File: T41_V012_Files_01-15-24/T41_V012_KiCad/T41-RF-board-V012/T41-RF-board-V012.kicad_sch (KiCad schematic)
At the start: 224 parts, among them J1 IQ_Out, J2 RF_IN, J3 RFControl, J4 12-13.8V, J5 IQ_In, J6 RF_OUT, Q1 BS170, U1 74CBTLV3253DR, U10 SN74LVC1G04DCK, U106 MC33078, U107 MC33078, U11 Si5351A-B-GT, U12 PE4312, U13 MAR-3SM+, U14 LM7805CT, U15 LM1117T-3.3, U16 MC33078, U17 LM317L, U18 SN74LVC1G04DCK, U19 MASWSS0179, U2 PSA-8A+, U20 MASWSS0179, U21 MCP23017_SO, U22 HMC434E, U23 HMC434E, U3 PE4312, U4 74CBTLV3253DR, U5 SN74LVC1G04DCK, U6 MC33078, U7 MASWSS0179, U8 MC33078, U9 MASWSS0179, Y1 ECS-TX053-S3, Y2 25MHz

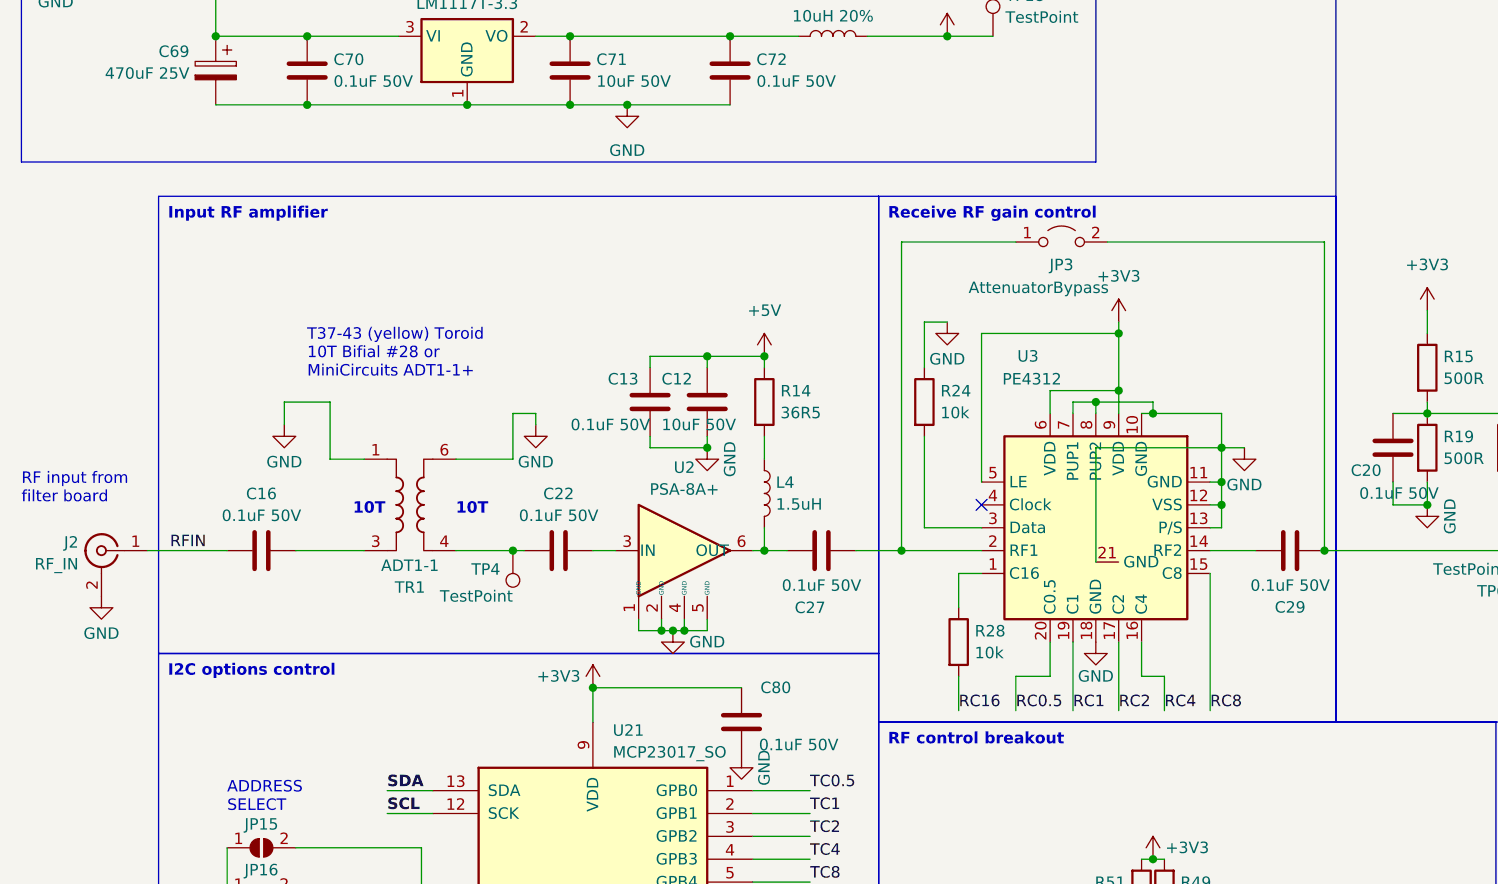
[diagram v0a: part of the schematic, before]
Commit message: Switched order of attenuator and amplifier in receive chain. Now attenuator is before amplifier
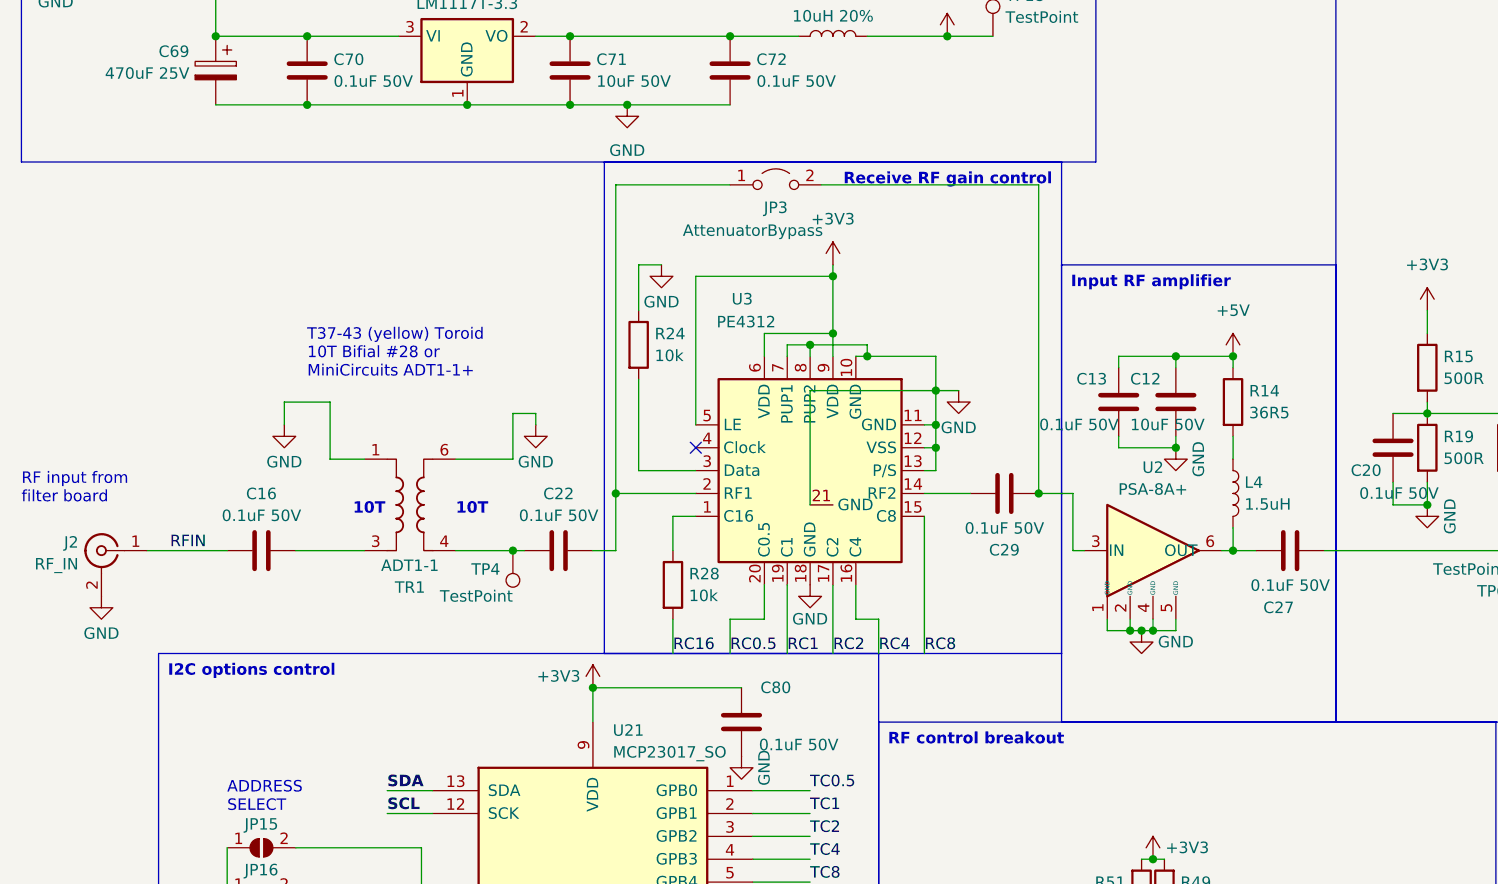
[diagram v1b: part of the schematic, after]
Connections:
- net at R20.2, TP6.1, U1.7 (1A)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: now also C27.2; no longer C29.2, JP3.2 (B)
- net at JP3.1 (A), U3.2 (RF1): now also C22.2; no longer C27.2
- net at U2.3 (IN): now also C29.2, JP3.2 (B); no longer C22.2
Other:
- moved on the sheet: C12, C13, C27, C29, JP3, L4, R14, R24, R28, U2, U3
